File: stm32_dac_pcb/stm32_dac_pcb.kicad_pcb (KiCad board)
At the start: 2 copper layers, 64.3 x 21.8 mm, 46 parts, among them J201 Conn_01x03, J202 Conn_01x05, J203 Conn_01x01, J301 AudioJack4, P201 USB_C_Plug_USB2.0, SW201 SW_Push, SW202 SW_Push, SW203 SW_Push, U101 AP1117-33, U102 AP1117-33, U201 STM32F411CEUx, U301 PCM5102A

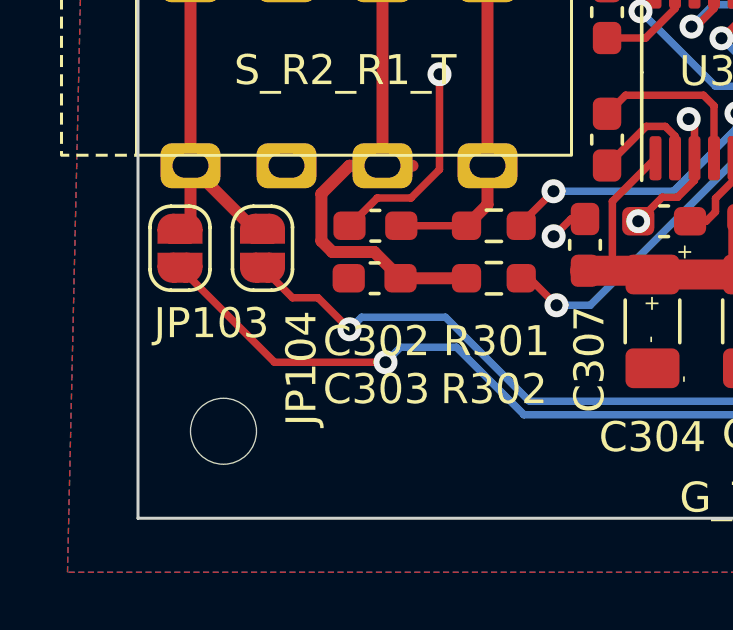
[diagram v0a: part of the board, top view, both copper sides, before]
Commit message: Small updates
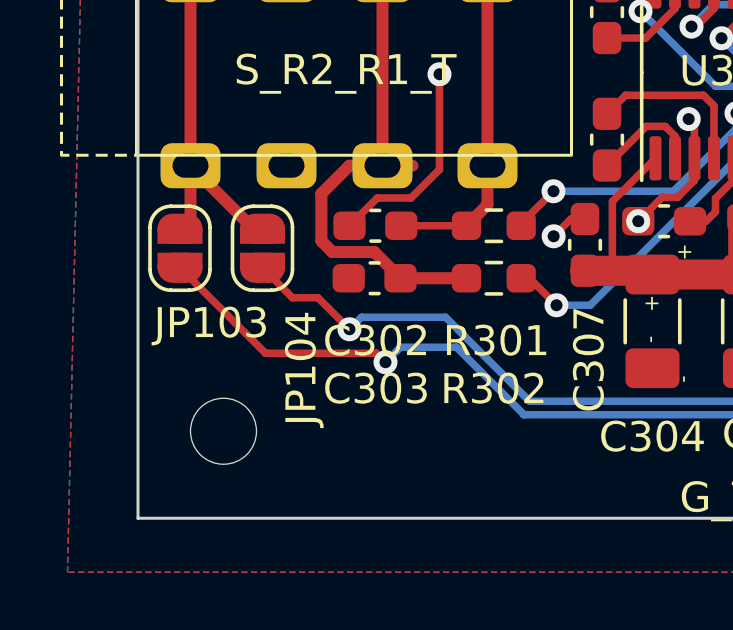
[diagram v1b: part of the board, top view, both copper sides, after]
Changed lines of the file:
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@@
   (segment (start 140.5625 102.17474) (end 140.5625 101.6875) (width 0.25) (layer "F.Cu") (net 52))
   (segment (start 139.983002 102.45) (end 140.28724 102.45) (width 0.25) (layer "F.Cu") (net 52))
+  (segment (start 104.1 101.8) (end 103.8 101.5) (width 0.25) (layer "F.Cu") (net 52))
   (segment (start 139.5 102.7755) (end 139.657502 102.7755) (width 0.25) (layer "F.Cu") (net 52))
   (segment (start 140.28724 102.45) (end 140.5625 102.17474) (width 0.25) (layer "F.Cu") (net 52))
-  (segment (start 100.4 101.8) (end 97.25 98.65) (width 0.25) (layer "F.Cu") (net 52))
-  (segment (start 104.1 101.8) (end 100.4 101.8) (width 0.25) (layer "F.Cu") (net 52))
+  (segment (start 103.8 101.5) (end 100.1 101.5) (width 0.25) (layer "F.Cu") (net 52))
+  (segment (start 100.1 101.5) (end 97.25 98.65) (width 0.25) (layer "F.Cu") (net 52))
   (segment (start 139.657502 102.7755) (end 139.983002 102.45) (width 0.25) (layer "F.Cu") (net 52))
   (via (at 104.1 101.8) (size 0.8) (drill 0.4) (layers "F.Cu" "B.Cu") (net 52))
